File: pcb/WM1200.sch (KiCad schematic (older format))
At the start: 0 parts

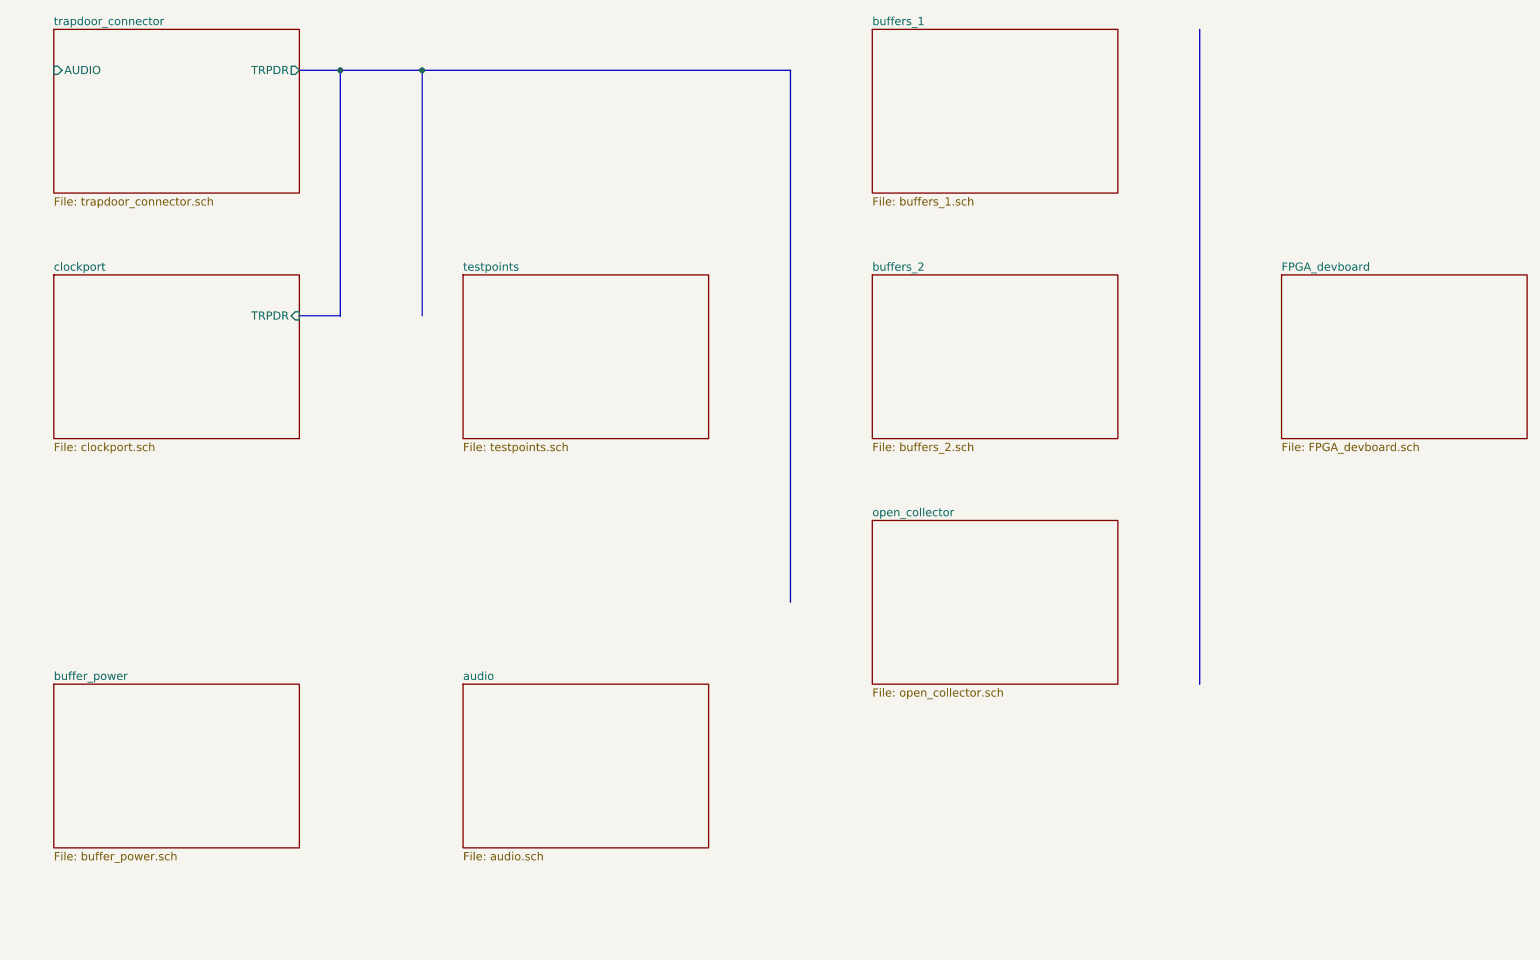
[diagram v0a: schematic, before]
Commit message: some work on sheets
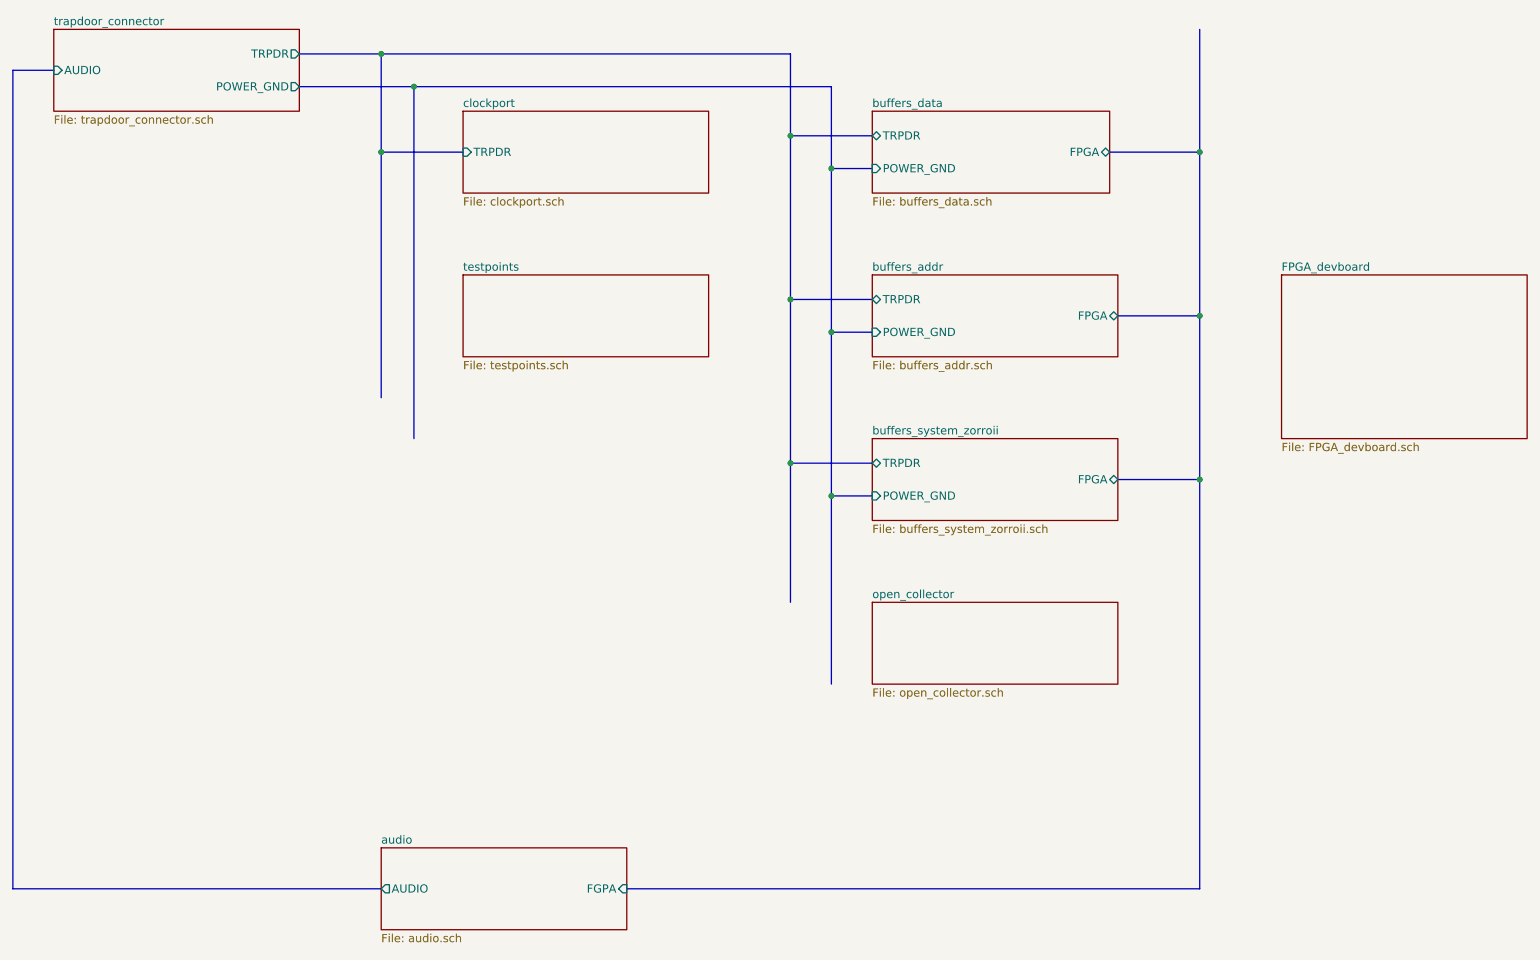
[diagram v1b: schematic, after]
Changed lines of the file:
@@
 $EndDescr
 $Sheet
-S 1000 1000 1500 1000
+S 1000 1000 1500 500
 U 5E6286C8
 F0 "trapdoor_connector" 50
 F1 "trapdoor_connector.sch" 50
-F2 "TRPDR" O R 2500 1250 50
+F2 "TRPDR" O R 2500 1150 50
 F3 "AUDIO" I L 1000 1250 50
+F4 "POWER_GND" O R 2500 1350 50
 $EndSheet
 $Sheet
-S 1000 2500 1500 1000
+S 3500 1500 1500 500
 U 5E55E8C3
 F0 "clockport" 50
 F1 "clockport.sch" 50
-F2 "TRPDR" I R 2500 2750 50
+F2 "TRPDR" I L 3500 1750 50
 $EndSheet
 Wire Bus Line
-	2500 1250 2750 1250
+	2500 1150 3000 1150
 $Sheet
-S 3500 2500 1500 1000
+S 3500 2500 1500 500
 U 5E5B86AA
 F0 "testpoints" 50
 F1 "testpoints.sch" 50
 $EndSheet
+Wire Bus Line
+	3000 1150 3000 1750
+Wire Bus Line
+	3000 1750 3500 1750
+Connection ~ 3000 1150
 $Sheet
-S 6000 1000 1500 1000
-U 5E5B89F7
-F0 "buffers_1" 50
-F1 "buffers_1.sch" 50
-$EndSheet
-$Sheet
-S 6000 2500 1500 1000
-U 5E5B8B5B
-F0 "buffers_2" 50
-F1 "buffers_2.sch" 50
-$EndSheet
-Wire Bus Line
-	2750 1250 2750 2750
-Wire Bus Line
-	2750 2750 2500 2750
-Connection ~ 2750 1250
-Wire Bus Line
-	2750 1250 3250 1250
-$Sheet
-S 6000 4000 1500 1000
+S 6000 4500 1500 500
 U 5E5B9D2E
 F0 "open_collector" 50
@@
 $EndSheet
 Wire Bus Line
-	3250 2750 3250 1250
-Connection ~ 3250 1250
+	5500 1150 5500 1650
 Wire Bus Line
-	5500 1250 5500 4500
-Wire Bus Line
-	3250 1250 5500 1250
-Wire Bus Line
-	8000 1000 8000 5000
+	8000 1000 8000 1750
 $Sheet
-S 1000 5000 1500 1000
-U 5E5BBEAC
-F0 "buffer_power" 50
-F1 "buffer_power.sch" 50
-$EndSheet
-$Sheet
-S 3500 5000 1500 1000
+S 3000 6000 1500 500
 U 5E5BC361
 F0 "audio" 50
 F1 "audio.sch" 50
+F2 "AUDIO" O L 3000 6250 50
+F3 "FGPA" I R 4500 6250 50
 $EndSheet
+$Sheet
+S 6000 1500 1450 500
+U 5E5B89F7
+F0 "buffers_data" 50
+F1 "buffers_data.sch" 50
+F2 "FPGA" B R 7450 1750 50
+F3 "TRPDR" B L 6000 1650 50
+F4 "POWER_GND" I L 6000 1850 50
+$EndSheet
+$Sheet
+S 6000 2500 1500 500
+U 5E78104B
+F0 "buffers_addr" 50
+F1 "buffers_addr.sch" 50
+F2 "FPGA" B R 7500 2750 50
+F3 "TRPDR" B L 6000 2650 50
+F4 "POWER_GND" I L 6000 2850 50
+$EndSheet
+$Sheet
+S 6000 3500 1500 500
+U 5E78B6EB
+F0 "buffers_system_zorroii" 50
+F1 "buffers_system_zorroii.sch" 50
+F2 "FPGA" B R 7500 3750 50
+F3 "TRPDR" B L 6000 3650 50
+F4 "POWER_GND" I L 6000 3850 50
+$EndSheet
+Wire Bus Line
+	1000 1250 750  1250
+Wire Bus Line
+	750  1250 750  6250
+Wire Bus Line
+	750  6250 3000 6250
+Wire Bus Line
+	3000 1150 5500 1150
+Connection ~ 3000 1750
+Wire Bus Line
+	3000 1750 3000 3250
+Wire Bus Line
+	5750 1350 5750 1850
+Wire Bus Line
+	2500 1350 3200 1350
+Wire Bus Line
+	5500 1650 6000 1650
+Connection ~ 5500 1650
+Wire Bus Line
+	5500 1650 5500 2650
+Wire Bus Line
+	6000 1850 5750 1850
+Connection ~ 5750 1850
+Wire Bus Line
+	5750 1850 5750 2850
+Wire Bus Line
+	6000 2650 5500 2650
+Connection ~ 5500 2650
+Wire Bus Line
+	6000 2850 5750 2850
+Connection ~ 5750 2850
+Wire Bus Line
+	5750 2850 5750 3850
+Wire Bus Line
+	6000 3650 5500 3650
+Wire Bus Line
+	5500 2650 5500 3650
+Connection ~ 5500 3650
+Wire Bus Line
+	5500 3650 5500 4500
+Wire Bus Line
+	6000 3850 5750 3850
+Connection ~ 5750 3850
+Wire Bus Line
+	5750 3850 5750 5000
+Wire Bus Line
+	3200 1350 3200 3500
+Connection ~ 3200 1350
+Wire Bus Line
+	3200 1350 5750 1350
+Wire Bus Line
+	7450 1750 8000 1750
+Connection ~ 8000 1750
+Wire Bus Line
+	7500 2750 8000 2750
+Wire Bus Line
+	8000 1750 8000 2750
+Connection ~ 8000 2750
+Wire Bus Line
+	8000 2750 8000 3750
+Wire Bus Line
+	7500 3750 8000 3750
+Connection ~ 8000 3750
+Wire Bus Line
+	4500 6250 8000 6250
+Wire Bus Line
+	8000 3750 8000 6250
 $EndSCHEMATC
